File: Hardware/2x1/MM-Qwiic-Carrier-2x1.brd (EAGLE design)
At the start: 106.7 x 35.6 mm, 88 parts, among them J15 MICROMOD-2222-C, J2 QWIIC_RIGHT_ANGLE, J5 Vertical Qwiic Connector, U1 MCP73831, U5 AP7361C-33FGEUDFN-8

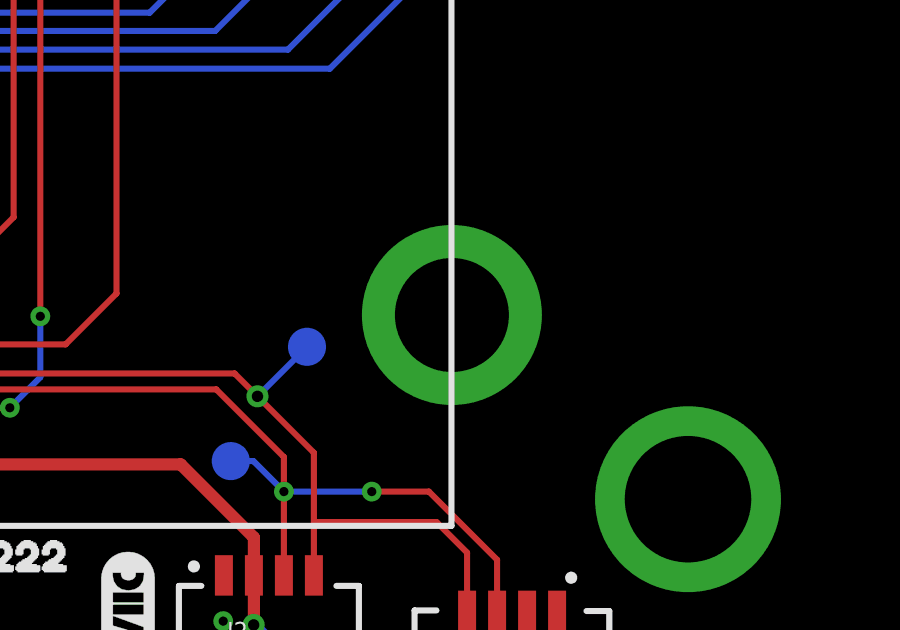
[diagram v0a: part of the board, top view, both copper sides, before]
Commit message: QC Feedback
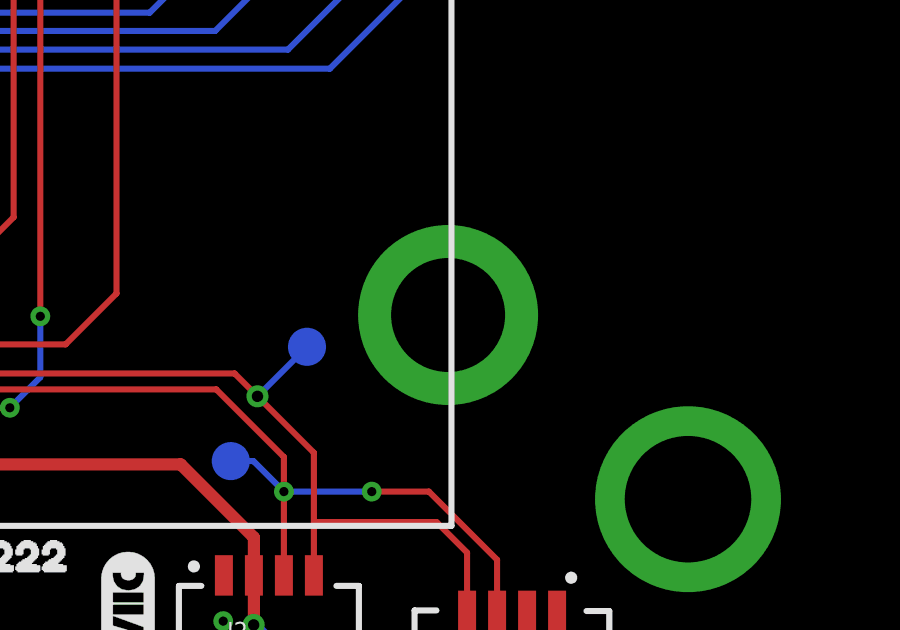
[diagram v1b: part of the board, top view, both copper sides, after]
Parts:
- moved H5 0.13 mm to (44.1, 13.8)
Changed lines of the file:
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@@
 <wire x1="44.185" y1="6.731" x2="27.94" y2="6.731" width="0.2032" layer="21"/>
 <text x="36.83" y="-21.59" size="1.778" layer="51" font="vector" ratio="15">Priyanka Makin</text>
-<text x="56.134" y="39.878" size="1.778" layer="47" font="vector" ratio="15">in</text>
-<text x="113.284" y="23.241" size="1.778" layer="47" font="vector" ratio="15" rot="R270">in</text>
-<text x="56.134" y="44.958" size="1.778" layer="47" font="vector" ratio="15">in</text>
+<text x="56.134" y="42.418" size="1.778" layer="47" font="vector" ratio="15">in</text>
+<text x="112.014" y="23.241" size="1.778" layer="47" font="vector" ratio="15" rot="R270">in</text>
+<text x="56.134" y="46.228" size="1.778" layer="47" font="vector" ratio="15">in</text>
 <text x="108.204" y="23.241" size="1.778" layer="47" font="vector" ratio="15" rot="R270">in</text>
-<dimension x1="2.54" y1="33.02" x2="104.14" y2="33.02" x3="53.34" y3="39.37" textsize="1.778" textratio="15" layer="47" unit="inch"/>
-<dimension x1="0" y1="35.56" x2="106.68" y2="35.56" x3="53.34" y3="44.45" textsize="1.778" textratio="15" layer="47" unit="inch"/>
-<dimension x1="104.14" y1="33.02" x2="104.14" y2="2.54" x3="110.49" y3="17.78" textsize="1.778" textratio="15" layer="47" unit="inch"/>
-<dimension x1="106.68" y1="35.56" x2="106.68" y2="0" x3="115.57" y3="17.78" textsize="1.778" textratio="15" layer="47" unit="inch"/>
+<dimension x1="2.54" y1="33.02" x2="104.14" y2="33.02" x3="53.34" y3="41.91" textsize="1.778" textratio="15" layer="47" unit="inch"/>
+<dimension x1="0" y1="35.56" x2="106.68" y2="35.56" x3="53.34" y3="45.72" textsize="1.778" textratio="15" layer="47" unit="inch"/>
+<dimension x1="104.14" y1="33.02" x2="104.14" y2="2.54" x3="114.3" y3="17.78" textsize="1.778" textratio="15" layer="47" unit="inch"/>
+<dimension x1="106.68" y1="35.56" x2="106.68" y2="0" x3="118.11" y3="17.78" textsize="1.778" textratio="15" layer="47" unit="inch"/>
+<dimension x1="81.28" y1="27.94" x2="101.6" y2="27.94" x3="91.44" y3="38.1" textsize="1.778" textratio="15" layer="47" unit="inch"/>
+<dimension x1="101.6" y1="27.94" x2="101.6" y2="7.62" x3="110.49" y3="17.78" textsize="1.778" textratio="15" layer="47" unit="inch"/>
+<text x="94.234" y="38.608" size="1.778" layer="47" font="vector" ratio="15">in</text>
+<text x="115.824" y="23.241" size="1.778" layer="47" font="vector" ratio="15" rot="R270">in</text>
 </plain>
 <attributes>
@@
 <element name="LOGO3" library="SparkFun-Aesthetics" package="OSHW-LOGO-M" value="OSHW-LOGOM" x="31.623" y="10.922" smashed="yes" rot="MR0"/>
 <element name="U$55" library="buzzard_labels (9)" package="22229" value="" x="26.962" y="5.72" smashed="yes"/>
-<element name="H5" library="SparkFun-Hardware" package="STAND-OFF-REFLOW-M2.5" value="STAND-OFF-REFLOW2.5MM_TALL" x="44.2" y="13.76" smashed="yes">
-<attribute name="PROD_ID" value="HW-14899" x="44.2" y="13.76" size="1.778" layer="27" font="vector" ratio="15" display="off"/>
+<element name="H5" library="SparkFun-Hardware" package="STAND-OFF-REFLOW-M2.5" value="STAND-OFF-REFLOW2.5MM_TALL" x="44.073" y="13.76" smashed="yes">
+<attribute name="PROD_ID" value="HW-14899" x="44.073" y="13.76" size="1.778" layer="27" font="vector" ratio="15" display="off"/>
 </element>
 <element name="JP4" library="SparkFun-Jumpers" package="SMT-JUMPER_2_NC_TRACE_SILK" package3d_urn="urn:adsk.eagle:package:39281/1" value="3V3 LED" x="15.24" y="33.655" smashed="yes" rot="MR0">
